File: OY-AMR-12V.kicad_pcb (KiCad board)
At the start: 2 copper layers, 21 parts, among them J1 34696-0100, K1 FBR51NL210-W1-RW, K2 FBR51ND12-W1, K3 FBR51ND12-W1, K4 FBR56ND12-W, K5 FBR56ND12-W

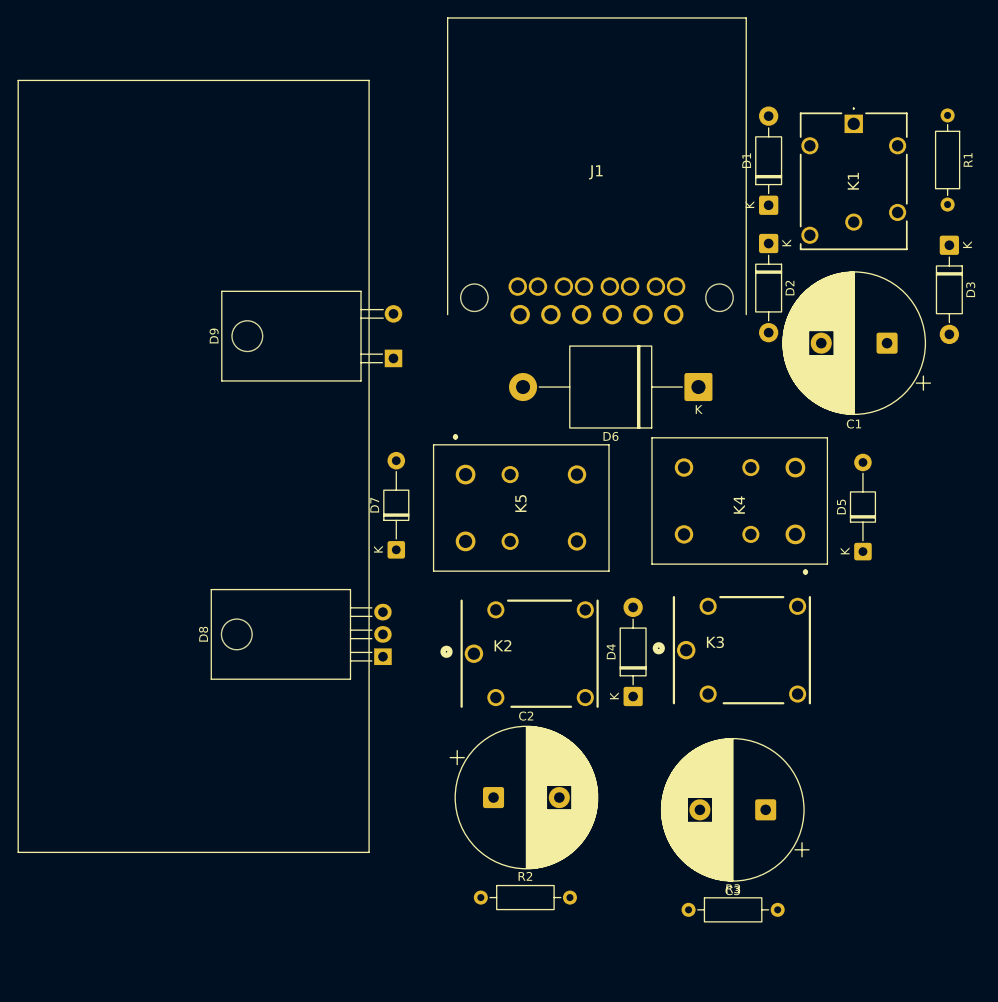
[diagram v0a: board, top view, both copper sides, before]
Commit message: PCB layout in progress
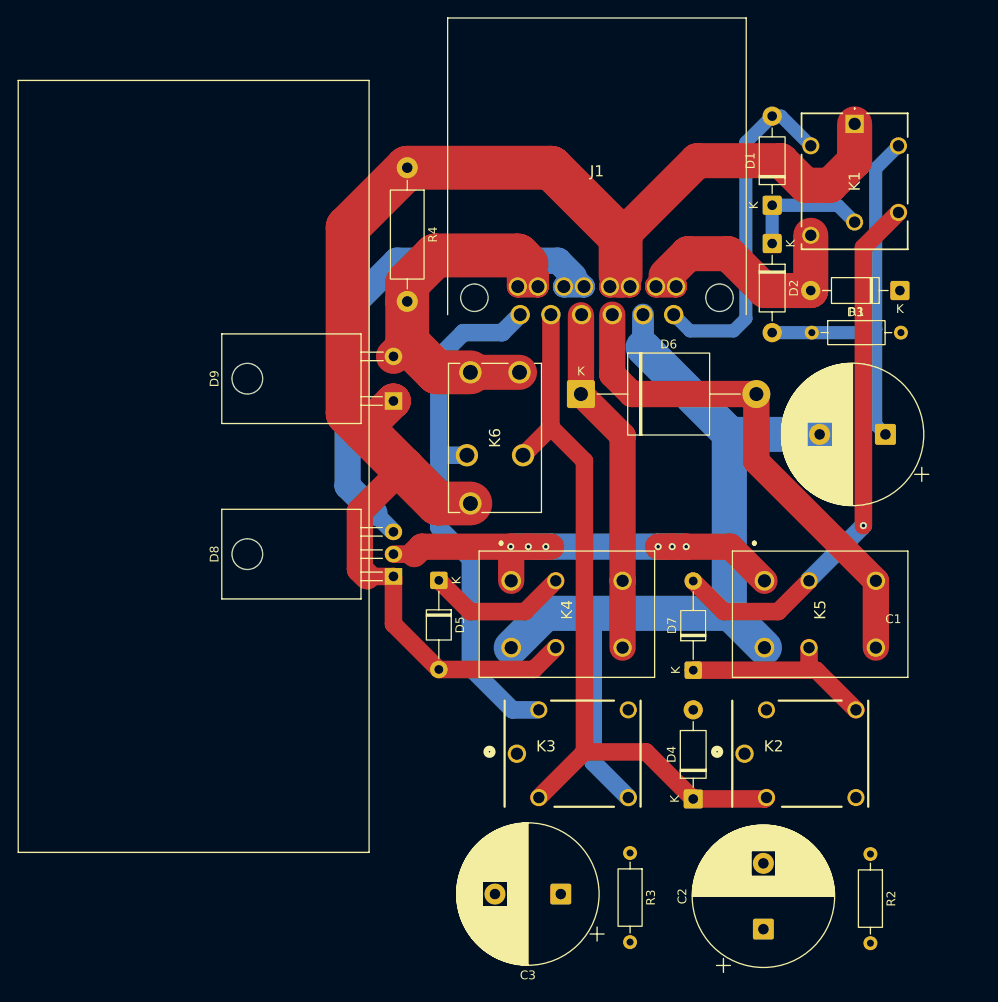
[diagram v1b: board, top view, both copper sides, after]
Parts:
- added K6: ACNH3212, SamacSys_Parts:ACNH3212, F.Cu at (122.8, 62.5)
- added R4: 47 2W, Resistor_THT:R_Axial_DIN0411_L9.9mm_D3.6mm_P15.24mm_Horizontal, F.Cu at (115.6, 39.2)
- D9: value FES16AT-E3/45 -> FES16AT
- moved D5 48.5 mm to (119.2, 86.2), turned to -90 degrees
- moved R2 44.7 mm to (168.4, 117.4), turned to -90 degrees
- moved D7 36.5 mm to (148.2, 96.5)
- moved K5 36.2 mm to (156.3, 86.3)
- moved C2 34.2 mm to (156.2, 126.0), turned to 90 degrees
- moved K2 32.9 mm to (160.4, 106.0)
- moved K4 32.8 mm to (127.5, 86.3), turned to -90 degrees
- moved R1 29.2 mm to (161.7, 58.0), turned to 0 degrees
- moved C3 25.3 mm to (133.1, 122.0)
- moved K3 22.6 mm to (134.4, 106.0)
- moved D4 13.5 mm to (148.2, 111.2)
- moved D6 13.4 mm to (135.4, 65.0), turned to 0 degrees
- moved C1 10.4 mm to (170.1, 69.6)
- moved R3 9.30 mm to (141.0, 117.3), turned to -90 degrees
- moved D8 9.23 mm to (114.0, 85.8)
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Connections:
- J1 pad 1: /COIL_RETURN -> /KS_IN
- J1 pad 2: /COIL_DRIVER -> GND
- J1 pad 3: Net-(D6-A1) -> Net-(D6-A2)
- J1 pad 4: Net-(D6-A2) -> Net-(D6-A1)
- J1 pad 5: /KS_IN -> /COIL_RETURN
- J1 pad 6: GND -> /COIL_DRIVER
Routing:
- net +12V_AUX: track 0.00 -> 173.1 mm
- net GND: track 0.00 -> 103.2 mm
- net /COIL_RETURN: track 0.00 -> 86.3 mm
- net Net-(D7-A2): track 0.00 -> 62.3 mm, vias 0 -> 1
- net +12V_BATT: track 0.00 -> 61.7 mm
- net /COIL_DRIVER: track 0.00 -> 60.9 mm
- net Net-(D6-A2): track 0.00 -> 58.7 mm
- net Net-(D8-A): track 0.00 -> 56.0 mm, vias 0 -> 6
- net +12V_DCDC: track 0.00 -> 46.9 mm
- net Net-(D2-A): track 0.00 -> 46.5 mm
- net Net-(D6-A1): track 0.00 -> 40.1 mm
- net /KS_IN: track 0.00 -> 39.7 mm
- net /KS_ON: track 0.00 -> 31.3 mm
- net Net-(D7-A1): track 0.00 -> 23.0 mm
- net Net-(D5-A1): track 0.00 -> 16.3 mm
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
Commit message: Initial PCB layout
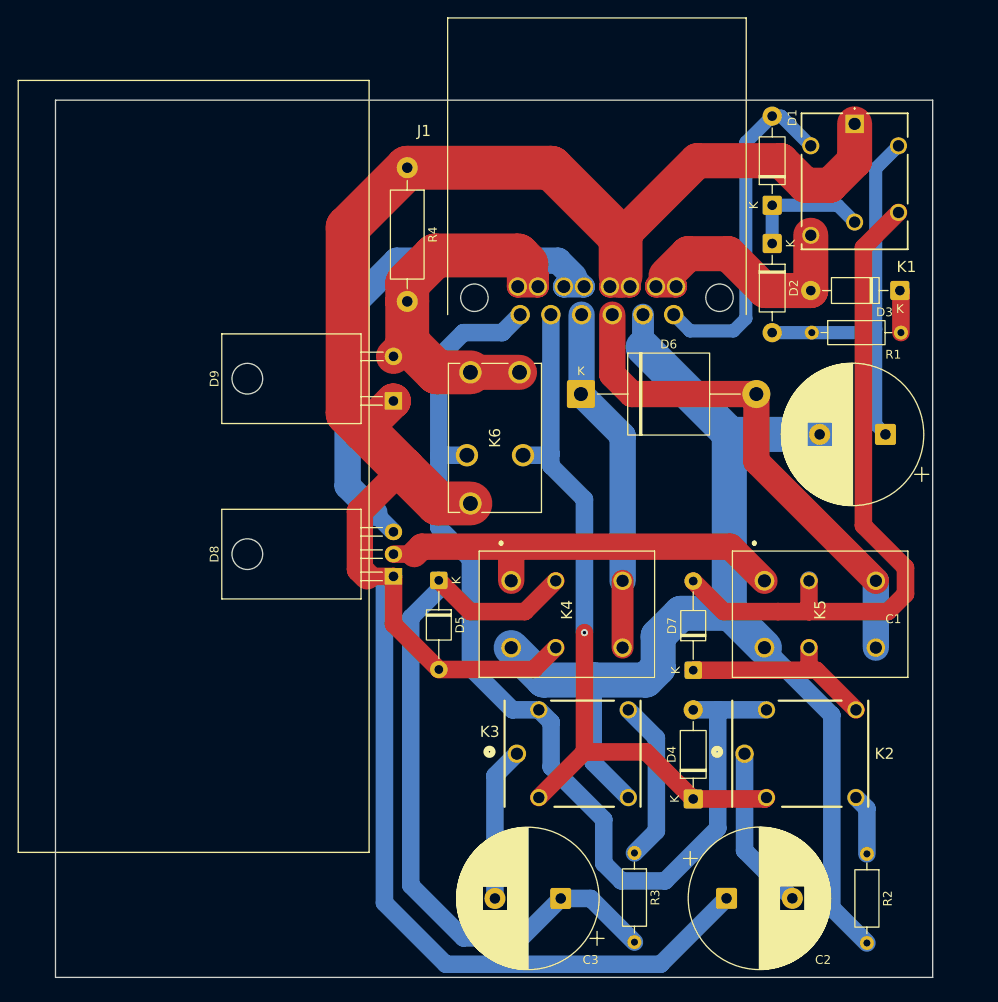
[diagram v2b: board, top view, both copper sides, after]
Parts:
- moved C2 5.48 mm to (152.0, 122.5), turned to 0 degrees
- moved C3 0.50 mm to (133.1, 122.5)
- moved R3 0.50 mm to (141.5, 117.3)
- moved R2 0.40 mm to (168.0, 117.4)
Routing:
- net +12V_AUX: track 173.1 -> 255.7 mm
- net Net-(D5-A1): track 16.3 -> 84.3 mm
- net /COIL_DRIVER: track 60.9 -> 119.6 mm
- net GND: track 103.2 -> 139.3 mm
- net Net-(C2-Pad2): track 0.00 -> 18.7 mm
- net Net-(K3-Pad4): track 0.00 -> 18.7 mm
- net Net-(C3-Pad2): track 0.00 -> 17.5 mm
- net Net-(D7-A2): track 62.3 -> 77.2 mm, vias 1 -> 0
- net Net-(D8-A): track 56.0 -> 48.1 mm, vias 6 -> 0
- net Net-(K2-Pad3): track 0.00 -> 6.94 mm
- net Net-(D3-K): track 0.00 -> 4.85 mm
- net /COIL_RETURN: track 86.3 -> 85.1 mm, vias 0 -> 1
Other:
- board outline added: 100 x 100 mm
